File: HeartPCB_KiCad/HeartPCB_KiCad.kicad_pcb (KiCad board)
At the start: 2 copper layers, 68.4 x 61 mm, 47 parts, among them J1 1051640001, J3 IN-, J4 IN+, J5 B+, J6 B-, Q1 FS8205A, U1 TP4056-42-ESOP8, U2 DW01A, U5 MCP4922

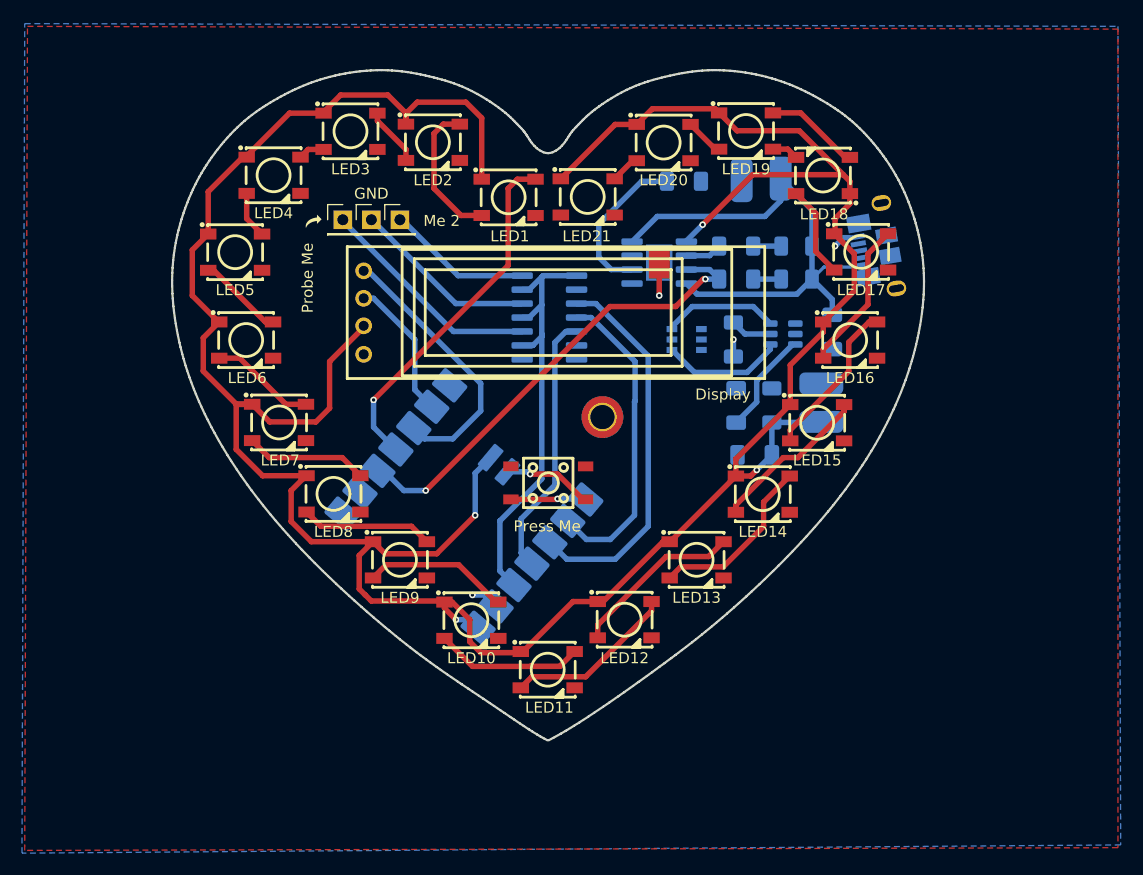
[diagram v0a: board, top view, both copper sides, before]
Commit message: final version for order
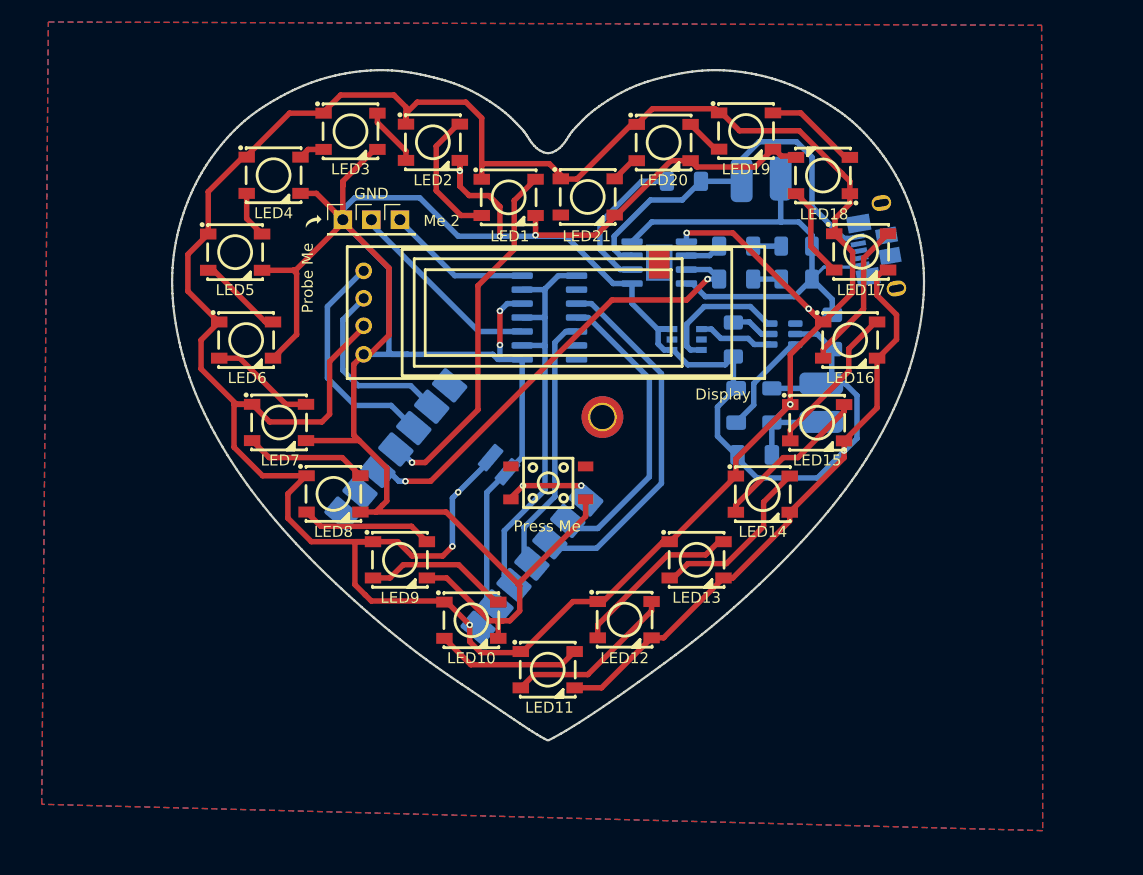
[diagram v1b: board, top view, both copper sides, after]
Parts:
- turned Q1 to 0 degrees
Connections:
- GND pad 1: GND -> Net-(J8-Pin_1)
- Probe Me pad 1: Net-(J8-Pin_1) -> GND
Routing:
- net GND: track 33.0 -> 394.0 mm, vias 4 -> 6
- net /V_BAT: track 268.5 -> 275.5 mm, vias 4 -> 6
- net Net-(U2-OD): track 11.1 -> 6.85 mm
- net Net-(U3-D5): track 13.0 -> 16.8 mm
- net Net-(U3-D4): track 24.9 -> 21.3 mm
- net unconnected-(U1-EPAD-Pad9): track 3.00 -> 0.00 mm, vias 1 -> 0
- net Net-(J8-Pin_1): track 20.4 -> 18.2 mm
- net Net-(U3-D7): track 6.86 -> 8.97 mm, vias 1 -> 2
- net Net-(U2-OC): track 10.6 -> 12.4 mm
- net Net-(U3-3V3): track 40.2 -> 38.5 mm
- net Net-(U3-D9): track 34.8 -> 33.2 mm
- net +5V_USB: track 48.2 -> 46.5 mm
- net /CHRG: track 43.1 -> 41.8 mm
- net Net-(U3-D8): track 28.7 -> 27.5 mm
- net /LED_Din: track 32.5 -> 33.6 mm
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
